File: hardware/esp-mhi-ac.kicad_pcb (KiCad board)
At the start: 2 copper layers, 89 x 40 mm, 15 parts, among them J1 CNS AC, J2 LS-HV, J3 LS-LV, J4 ADA BMEx80, J5 BMEx80, J6 BH1750, U1 WeMos_D1_mini, U2 TSR_1-2450

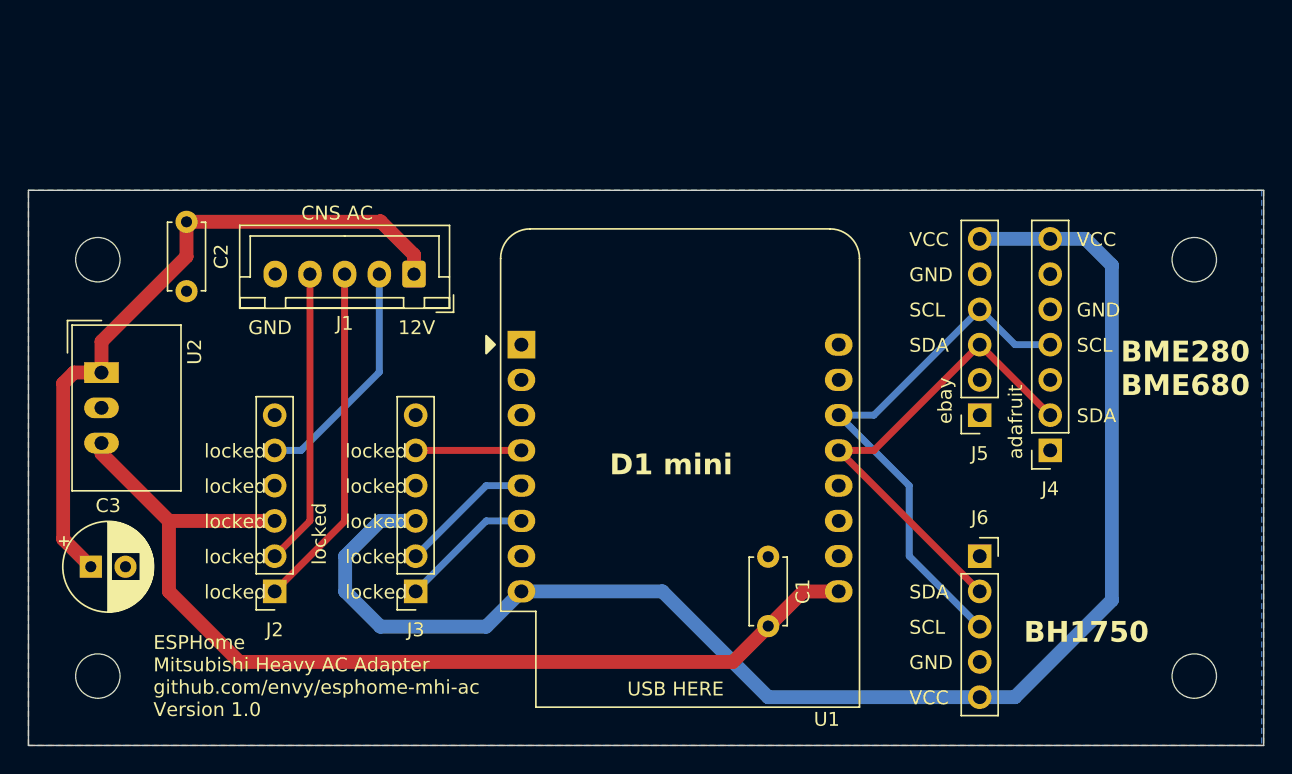
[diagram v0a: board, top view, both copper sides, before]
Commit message: update hardware
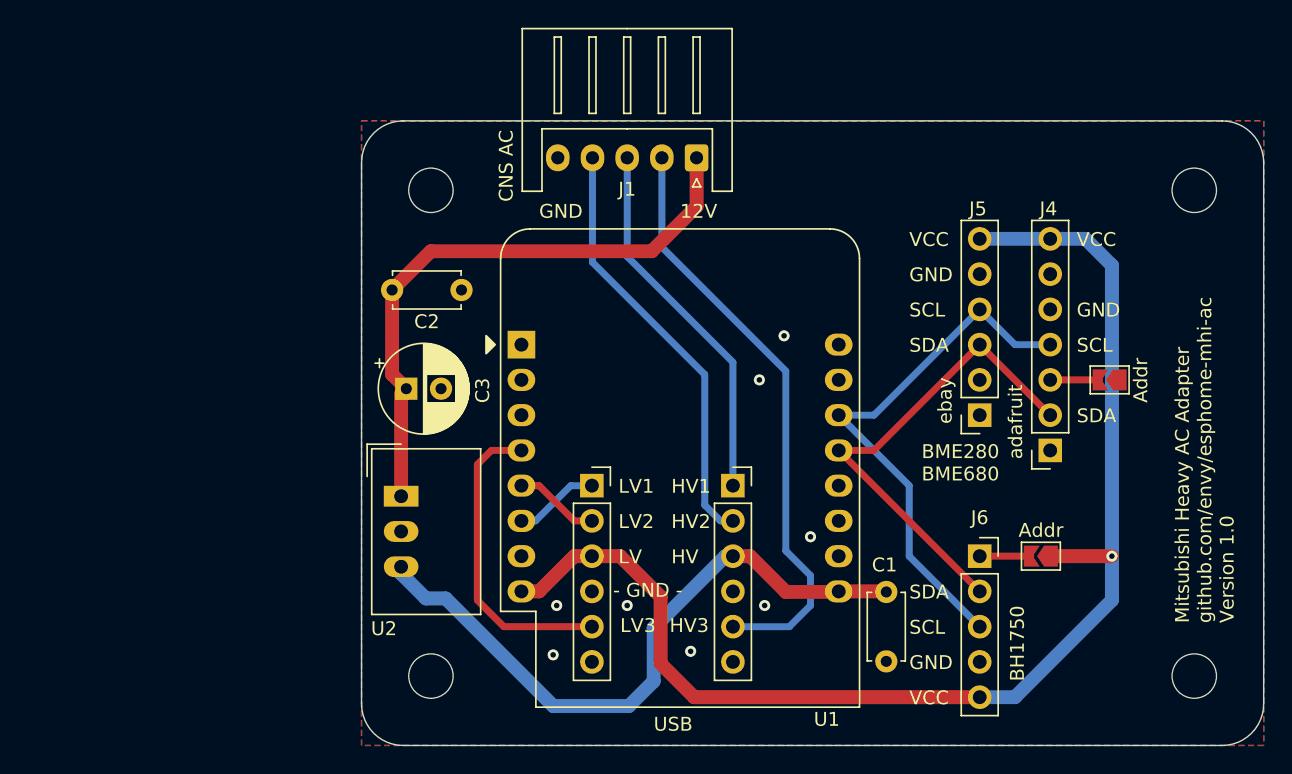
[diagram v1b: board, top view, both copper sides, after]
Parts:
- added JP1: BME680 ADDR, Jumper:SolderJumper-2_P1.3mm_Open_TrianglePad1.0x1.5mm, F.Cu at (138.9, 73.7)
- added JP2: BH1750 ADDR, Jumper:SolderJumper-2_P1.3mm_Open_TrianglePad1.0x1.5mm, F.Cu at (133.9, 86.4)
- J1: footprint Connector_JST:JST_XH_B5B-XH-A_1x05_P2.50mm_Vertical -> Connector_JST:JST_XH_S5B-XH-A_1x05_P2.50mm_Horizontal
- moved J2 33.9 mm to (111.8, 81.3), turned to 0 degrees
- moved C3 26.1 mm to (88.2, 74.3)
- moved H3 24.5 mm to (90.0, 60.0)
- moved H4 24.0 mm to (90.0, 95.0)
- moved U2 23.4 mm to (87.9, 82.0)
- moved J1 22.0 mm to (109.1, 57.7)
- moved C2 15.6 mm to (87.2, 67.2), turned to 0 degrees
- moved J3 14.8 mm to (101.6, 81.3), turned to 0 degrees
- moved C1 11.4 mm to (122.8, 93.9), turned to 90 degrees
- moved H1 5.00 mm to (145.0, 60.0)
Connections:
- J4 pad 3: unconnected-(J4-Pin_3-Pad3) -> Net-(J4-Pin_3)
- J6 pad 1: unconnected-(J6-Pin_1-Pad1) -> Net-(J6-Pin_1)
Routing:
- net HV3: track 16.9 -> 42.9 mm
- net +5V: track 72.8 -> 47.2 mm
- net LV3: track 7.62 -> 22.4 mm
- net +3.3V: track 106.5 -> 92.4 mm, vias 0 -> 1
- net HV2: track 21.4 -> 30.9 mm
- net +12V: track 50.1 -> 43.4 mm
- net Net-(J6-Pin_1): track 0.00 -> 3.68 mm
- net LV1: track 9.72 -> 6.13 mm
- net LV2: track 9.72 -> 6.13 mm
- net Net-(J4-Pin_3): track 0.00 -> 3.56 mm
- net HV1: track 25.0 -> 26.8 mm
- net GND: vias 0 -> 8
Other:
- board size 89 x 40 mm -> 65 x 45 mm
- board text added: "- GND -"
- board text added: "Addr"
- board text added: "HV"
- board text added: "HV1"
- board text added: "HV2"
- board text added: "HV3"
- board text added: "JLCJLCJLCJLC"
- board text added: "LV"
- board text added: "LV1"
- board text added: "LV2"
- board text added: "LV3"
- board text added: "Mitsubishi Heavy AC Adapter github.com/envy/esphome-mhi-ac Version 1.0"
- board text added: "USB"
- board text removed: "D1 mini"
- board text removed: "ESPHome Mitsubishi Heavy AC Adapter github.com/envy/esphome-mhi-ac Version 1.0"
- board text removed: "USB HERE"
- board text removed: "locked"
